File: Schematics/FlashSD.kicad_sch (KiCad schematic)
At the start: 3 parts, among them J3 Micro_SD_Card

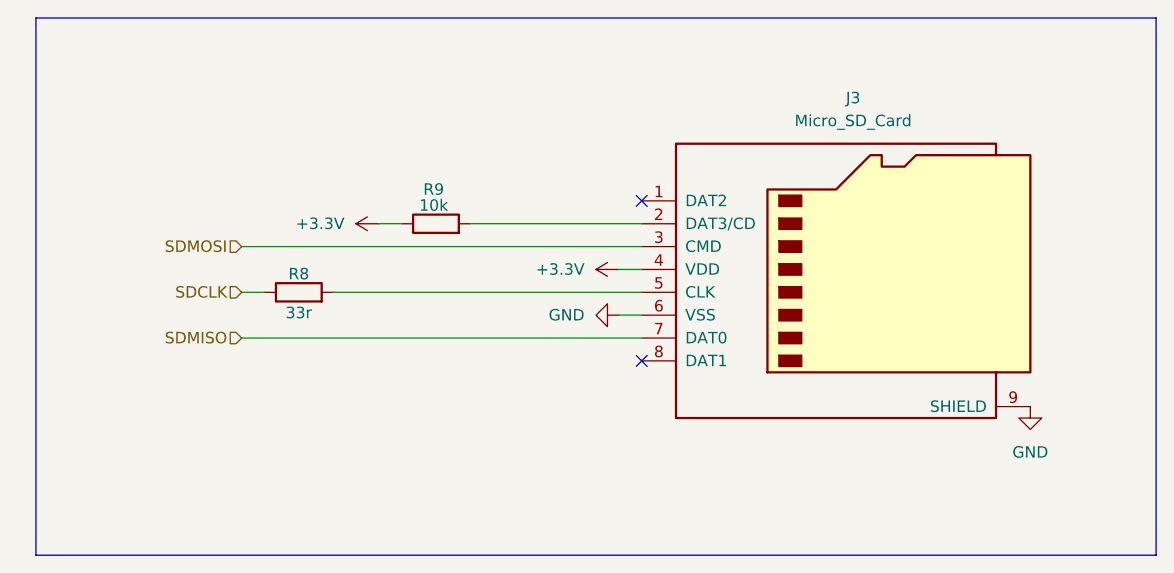
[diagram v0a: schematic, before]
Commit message: pcb pending review and order
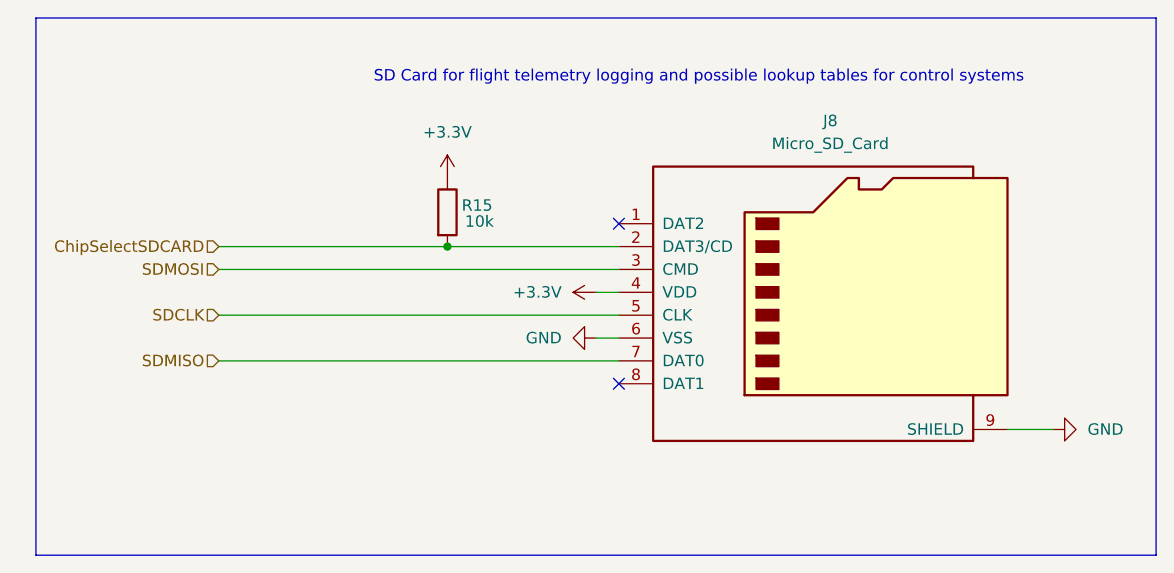
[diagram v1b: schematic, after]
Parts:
- removed J3: Micro_SD_Card, Connector_Card:microSD_HC_Molex_47219-2001, symbol Connector:Micro_SD_Card
- removed R8: 33r, Resistor_SMD:R_0805_2012Metric_Pad1.20x1.40mm_HandSolder, symbol Device:R
- removed R9: 10k, Resistor_SMD:R_0805_2012Metric_Pad1.20x1.40mm_HandSolder, symbol Device:R
- added J8: Micro_SD_Card, Connector_Card:microSD_HC_Molex_47219-2001, symbol Connector:Micro_SD_Card
- added R15: 10k, Resistor_SMD:R_0805_2012Metric_Pad1.20x1.40mm_HandSolder, symbol Device:R
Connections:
- net +3.3V: now also J8.4 (VDD), R15.1
- net GND: now also J8.6 (VSS), J8.9 (SHIELD)
- net SDCLK: now also J8.5 (CLK)
- net SDMISO: now also J8.7 (DAT0)
- net SDMOSI: now also J8.3 (CMD)
- new net ChipSelectSDCARD: J8.2 (DAT3/CD), R15.2
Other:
- note added: "SD Card for flight telemetry logging and possible lookup tables for control systems"
